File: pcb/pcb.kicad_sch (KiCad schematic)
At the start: 2 parts, among them CN1 1x3, SW1 switch_3x6

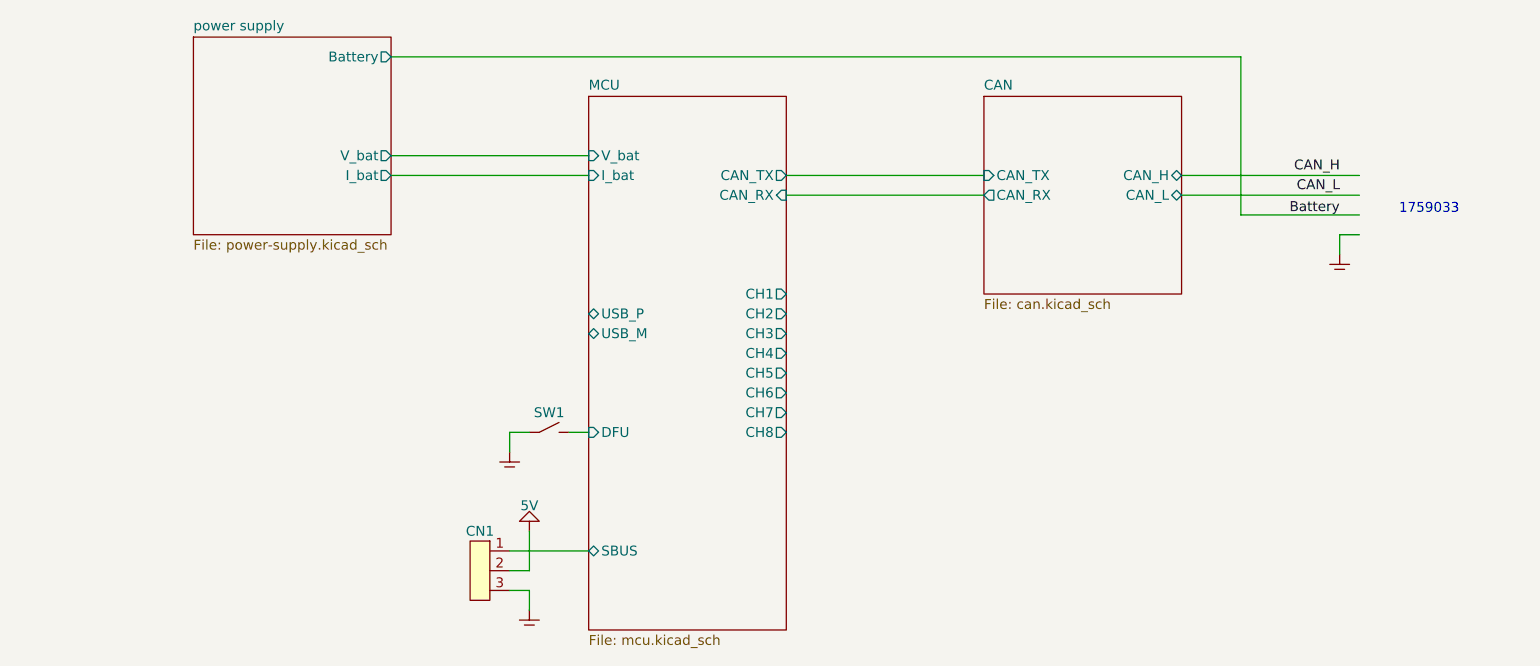
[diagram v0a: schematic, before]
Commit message: continued work on schematic
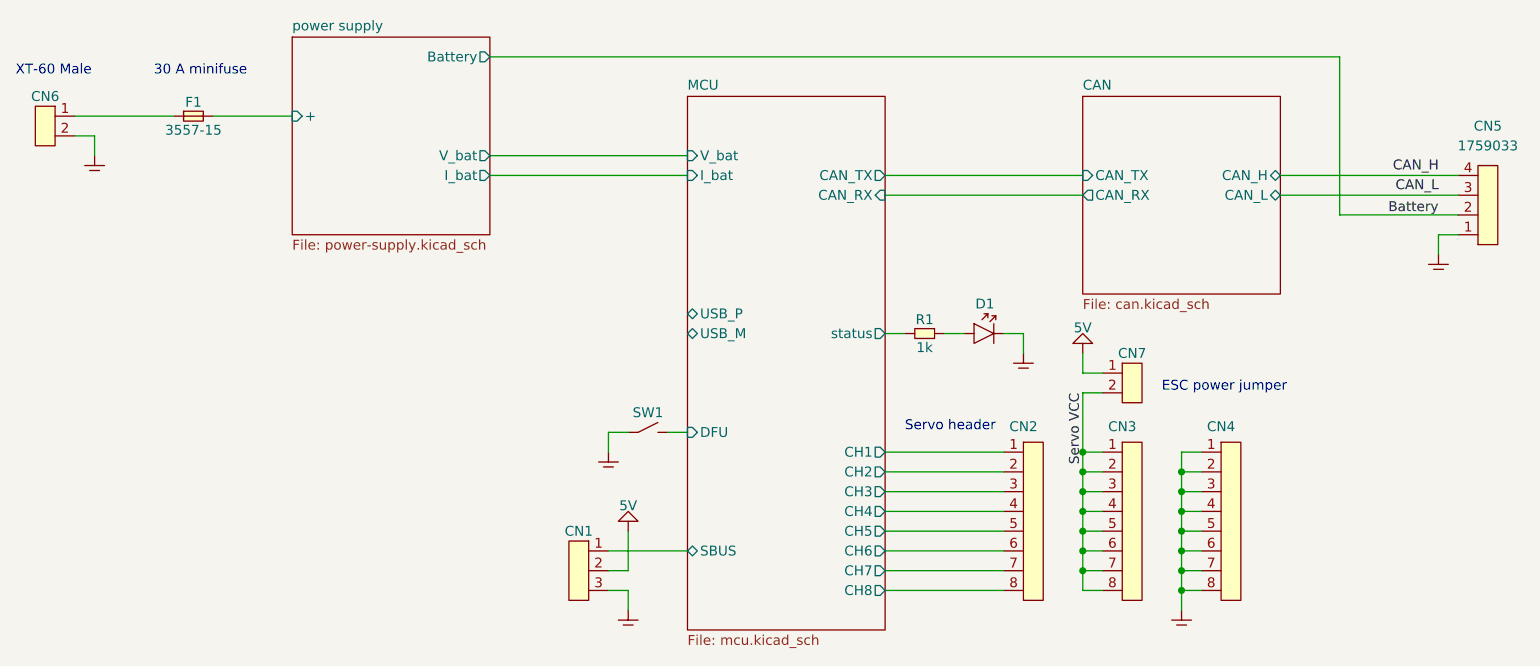
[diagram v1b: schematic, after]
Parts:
- added CN2, CN3, CN4: 1x8, symbol pin_headers:1x8
- added CN5: 1x4, symbol pin_headers:1x4
- added CN6, CN7: 1x2, symbol pin_headers:1x2
- added D1: LED, SMT:0603, symbol generic:LED
- added F1: F, SMT:0603, symbol generic:fuse
- added R1: 1k, SMT:0603, symbol generic:R
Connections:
- net Battery: now also CN5.2
- net CAN/CAN_H: now also CN5.4
- net CAN/CAN_L: now also CN5.3
- net GND: now also CN4.1, CN4.2, CN4.3, CN4.4, CN4.5, CN4.6, CN4.7, CN4.8, CN5.1, CN6.2, CN7.1, D1.2 (K)
- net MCU/CH1: now also CN2.1
- net MCU/CH2: now also CN2.2
- net MCU/CH3: now also CN2.3
- net MCU/CH4: now also CN2.4
- net MCU/CH5: now also CN2.5
- net MCU/CH6: now also CN2.6
- net MCU/CH7: now also CN2.7
- net MCU/CH8: now also CN2.8
- new net: D1.1 (A), R1.1
- new net: CN6.1, F1.1
- new net MCU/status: R1.2
- new net Servo VCC: CN3.1, CN3.2, CN3.3, CN3.4, CN3.5, CN3.6, CN3.7, CN3.8, CN7.2
- new net power supply/+: F1.2
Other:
- sheet MCU ports: added status; removed none
- sheet power supply ports: added +; removed none
- note added: "30 A minifuse"
- note added: "ESC power jumper"
- note added: "Servo header"
- note added: "XT-60 Male"
- note removed: "1759033"
- moved on the sheet: CN1, SW1
